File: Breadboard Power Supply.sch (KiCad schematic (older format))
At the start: 15 parts, among them J1 Barrel_Jack_Switch, J2 Conn_02x02_Odd_Even, J3 Conn_02x02_Odd_Even, SW1 SW_DPDT_x2, U1 LM7805_TO220

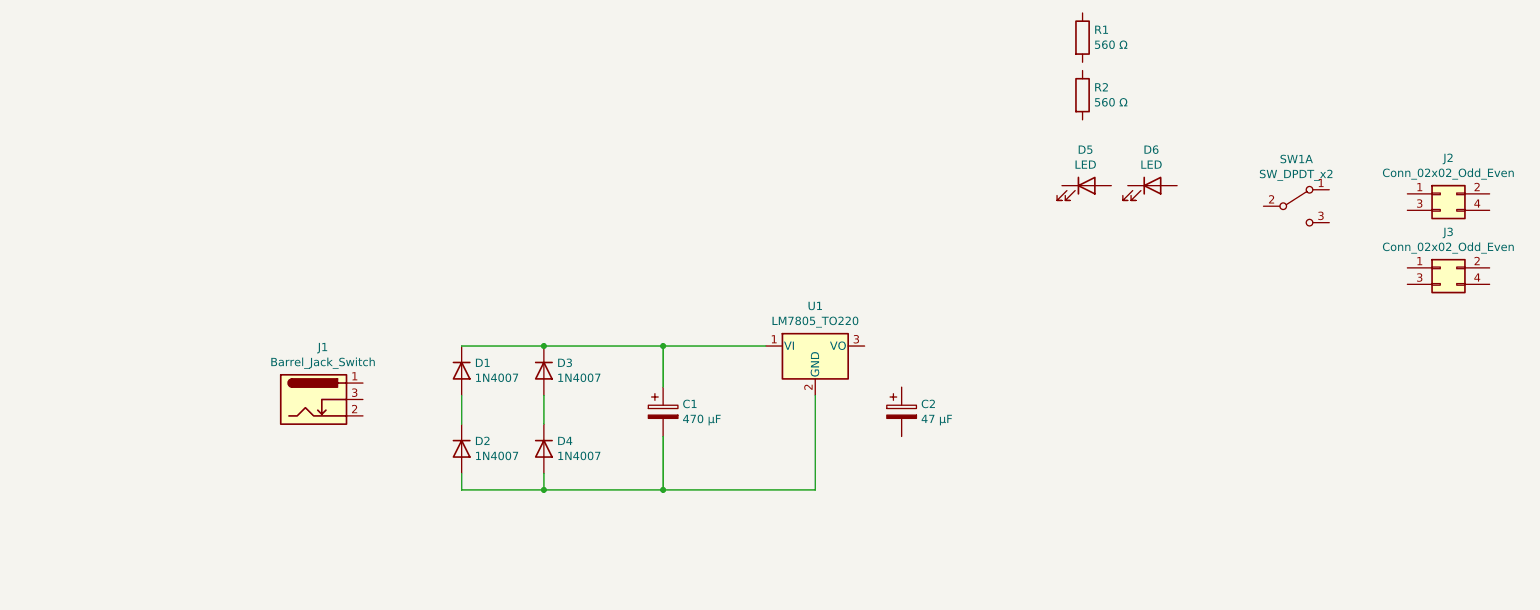
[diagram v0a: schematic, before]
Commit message: 101. video bitti
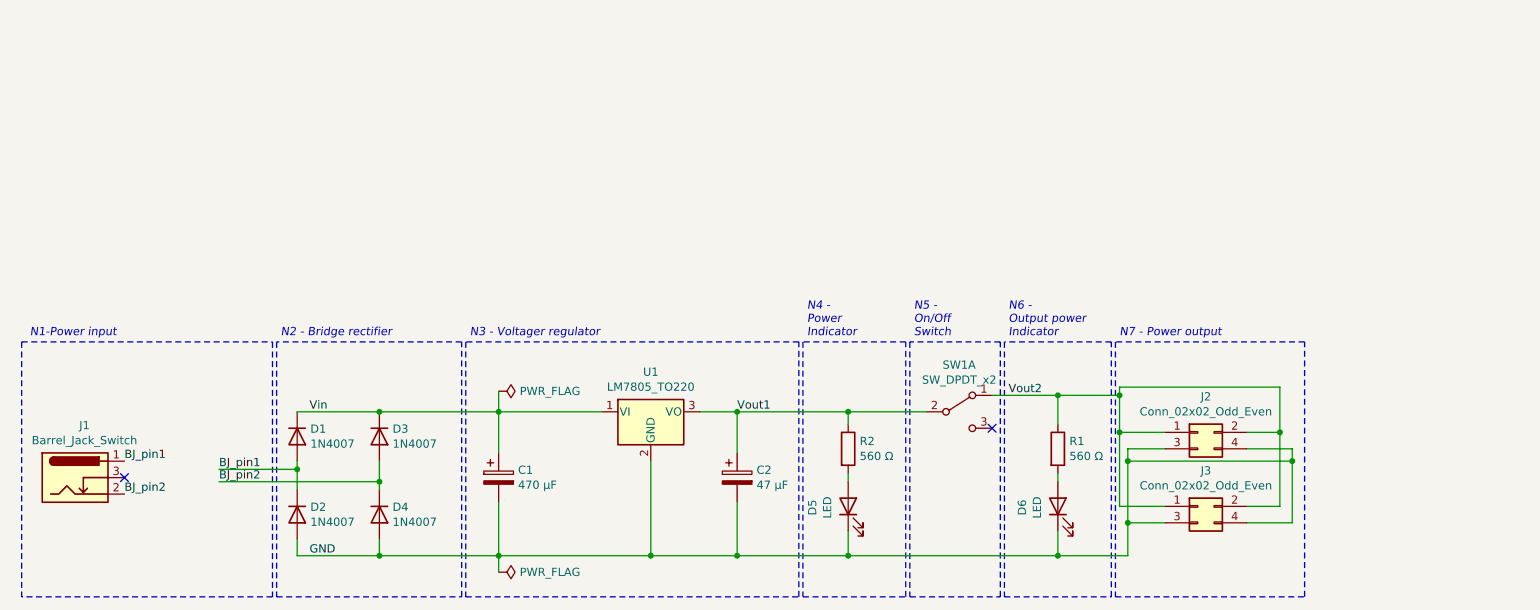
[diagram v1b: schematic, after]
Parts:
- J1: footprint Connector_PinHeader_2.54mm:PinHeader_1x28_P2.54mm_Vertical -> Connector_BarrelJack:BarrelJack_CUI_PJ-102AH_Horizontal
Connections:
- net Vout1: now reaches C2.1
- net Vout1: now also R2.1, SW1.2 (B), U1.3 (VO)
- net GND: now reaches C2.2
- net GND: now also C1.2, D2.2 (A), D4.2 (A), D5.1 (K), D6.1 (K), J2.3 (Pin_3), J2.4 (Pin_4), J3.3 (Pin_3), J3.4 (Pin_4), U1.2 (GND)
- net Vin: now reaches C1.1, D1.1 (K), D3.1 (K), U1.1 (VI)
- net Vout2: now reaches R1.1
- net Vout2: now also J2.1 (Pin_1), J2.2 (Pin_2), J3.1 (Pin_1), J3.2 (Pin_2), SW1.1 (A)
- net at R1.2: now also D6.2 (A)
- net at R2.2: now also D5.2 (A)
- net BJ_pin1: now reaches D1.2 (A), D2.1 (K)
- net BJ_pin1: now also J1.1
- net BJ_pin2: now reaches D3.2 (A), D4.1 (K)
- net BJ_pin2: now also J1.2
- no-connect marks 0 -> 2
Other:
- note added: "N1-Power input"
- note added: "N2 - Bridge rectifier"
- note added: "N3 - Voltager regulator"
- note added: "N4 - \nPower\nIndicator"
- note added: "N5 - \nOn/Off \nSwitch"
- note added: "N6 - \nOutput power\nIndicator"
- note added: "N7 - Power output"
- moved on the sheet: C1, C2, D1, D2, D3, D4, D5, D6, J1, J2, J3, R1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

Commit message: 104. video tamamlandı
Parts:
- C1, C2: symbol Device:C_Polarized -> Breadboard-Power-Supply-rescue:C_Polarized-Device
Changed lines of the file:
@@
 $EndDescr
 $Comp
-L Device:C_Polarized C2
+L Breadboard-Power-Supply-rescue:C_Polarized-Device C2
 U 1 1 612CFBC3
 P 5775 3725
@@
 $EndComp
 $Comp
-L Device:C_Polarized C1
+L Breadboard-Power-Supply-rescue:C_Polarized-Device C1
 U 1 1 612D6354
 P 4325 3725
